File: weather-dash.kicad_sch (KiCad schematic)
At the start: 7 parts, among them J1 Conn_01x02_Pin, J3 Conn_01x03_Socket, SW1 SW_Push, U1 WEMOS_C3_Mini, U2 TFT_ST7735_SD

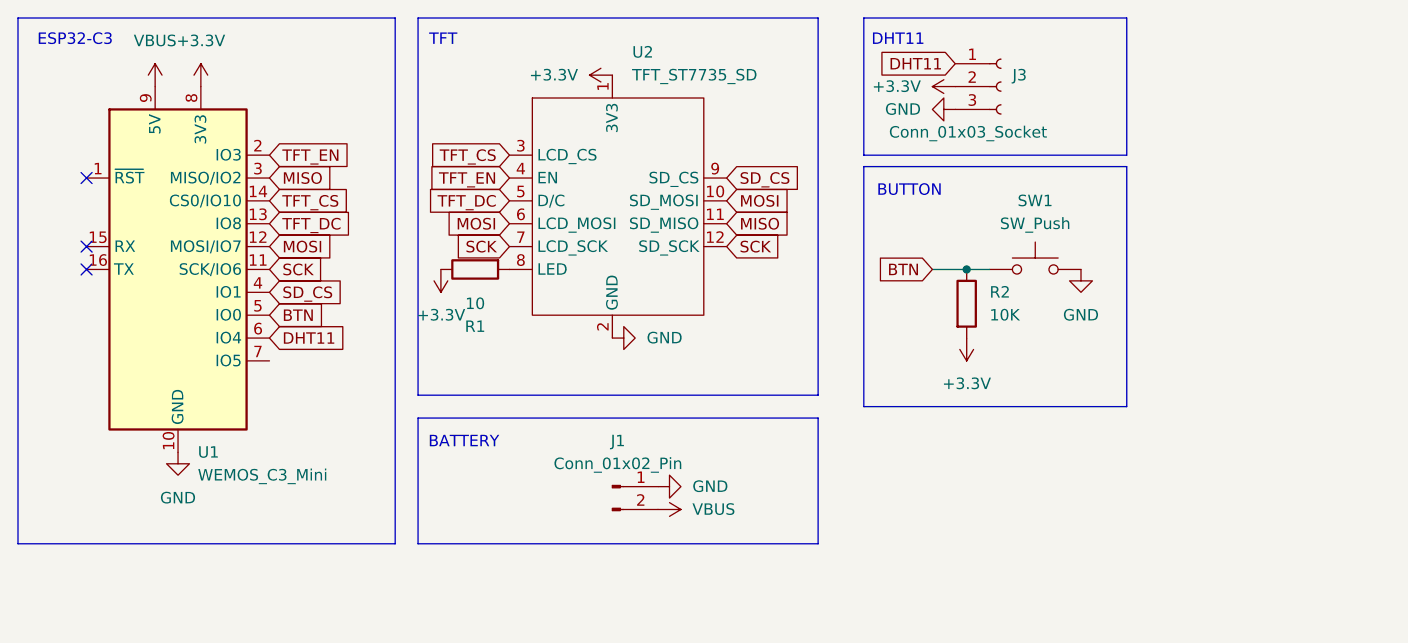
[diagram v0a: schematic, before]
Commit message: updates
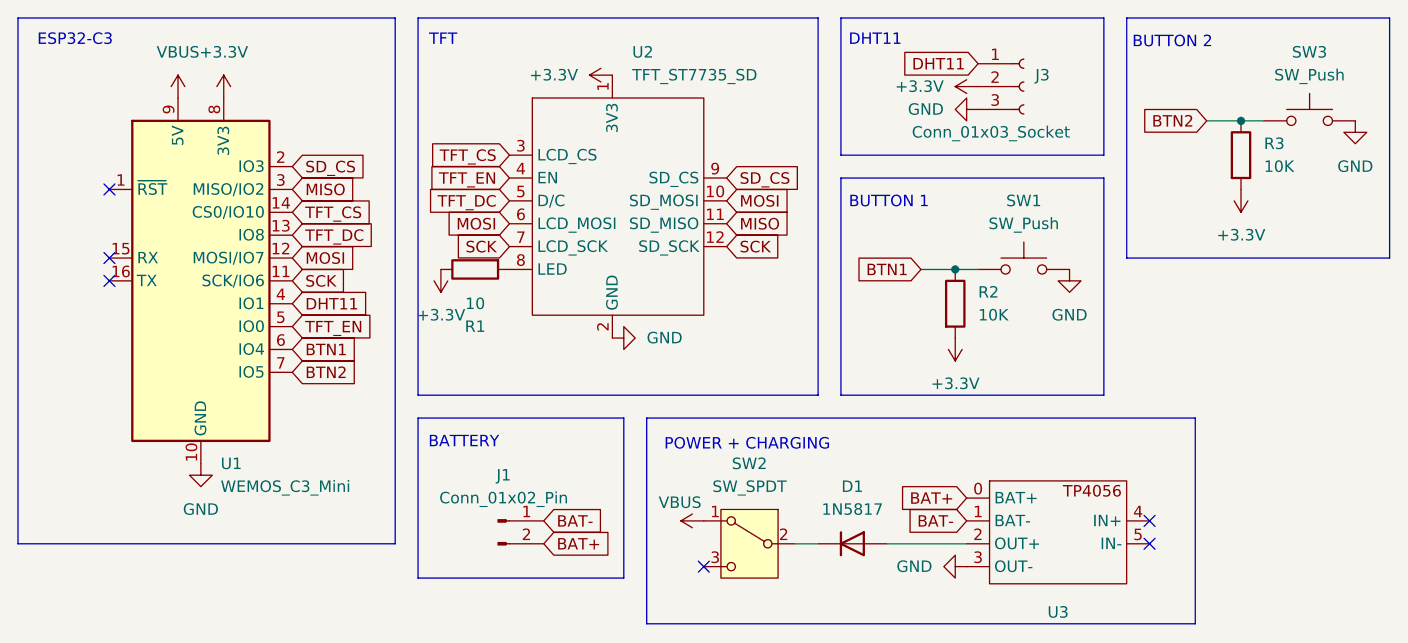
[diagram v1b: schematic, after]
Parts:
- added D1: 1N5817, Diode_THT:D_DO-41_SOD81_P7.62mm_Horizontal, symbol Device:D
- added R3: 10K, Resistor_THT:R_Axial_DIN0207_L6.3mm_D2.5mm_P7.62mm_Horizontal, symbol Device:R
- added SW2: SW_SPDT, Connector_JST:JST_PH_B2B-PH-K_1x02_P2.00mm_Vertical, symbol Switch:SW_SPDT
- added SW3: SW_Push, Button_Switch_THT:SW_PUSH_6mm_H4.3mm, symbol Switch:SW_Push
- added U3: ~, asylum-weather:TP4056, symbol asylum-weather:TP4056
- J3: footprint Connector_PinSocket_2.54mm:PinSocket_1x03_P2.54mm_Vertical -> asylum-weather:DHT11
- U1: footprint Module:WEMOS_D1_mini_light -> asylum-weather:WEMOS_C3_mini
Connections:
- net +3.3V: now also R3.2
- net DHT11: now also U1.4 (IO1); no longer U1.6 (IO4)
- net GND: now also SW3.2, U3.3 (OUT-); no longer J1.1 (Pin_1)
- net SD_CS: now also U1.2 (IO3); no longer U1.4 (IO1)
- net TFT_EN: now also U1.5 (IO0); no longer U1.2 (IO3)
- net VBUS: now also SW2.1 (A); no longer J1.2 (Pin_2)
- net BTN2: now reaches U1.7 (IO5)
- net BTN2: now also R3.1, SW3.1
- net BTN renamed BTN1
- net BTN1: now also U1.6 (IO4); no longer U1.5 (IO0)
- new net: D1.1 (K), SW2.2 (B)
- new net: D1.2 (A), U3.2 (OUT+)
- new net BAT+: J1.2 (Pin_2), U3.0 (BAT+)
- new net BAT-: J1.1 (Pin_1), U3.1 (BAT-)
- no-connect marks 3 -> 6
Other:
- note added: "BUTTON 1"
- note added: "BUTTON 2"
- note added: "POWER + CHARGING"
- note removed: "BUTTON"
- moved on the sheet: J1, J3, R2, SW1, U1
